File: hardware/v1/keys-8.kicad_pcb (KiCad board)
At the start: 2 copper layers, 13 parts, among them P1 CONN_02X02, P2 CONN_01X03, P3 CONN_01X03, P4 CONN_01X03, SW1 SWITCH_INV, SW2 SWITCH_INV, SW3 SWITCH_INV, SW4 SWITCH_INV, SW5 SWITCH_INV, SW6 SWITCH_INV, SW7 SWITCH_INV, SW8 SWITCH_INV, U1 MCP23017

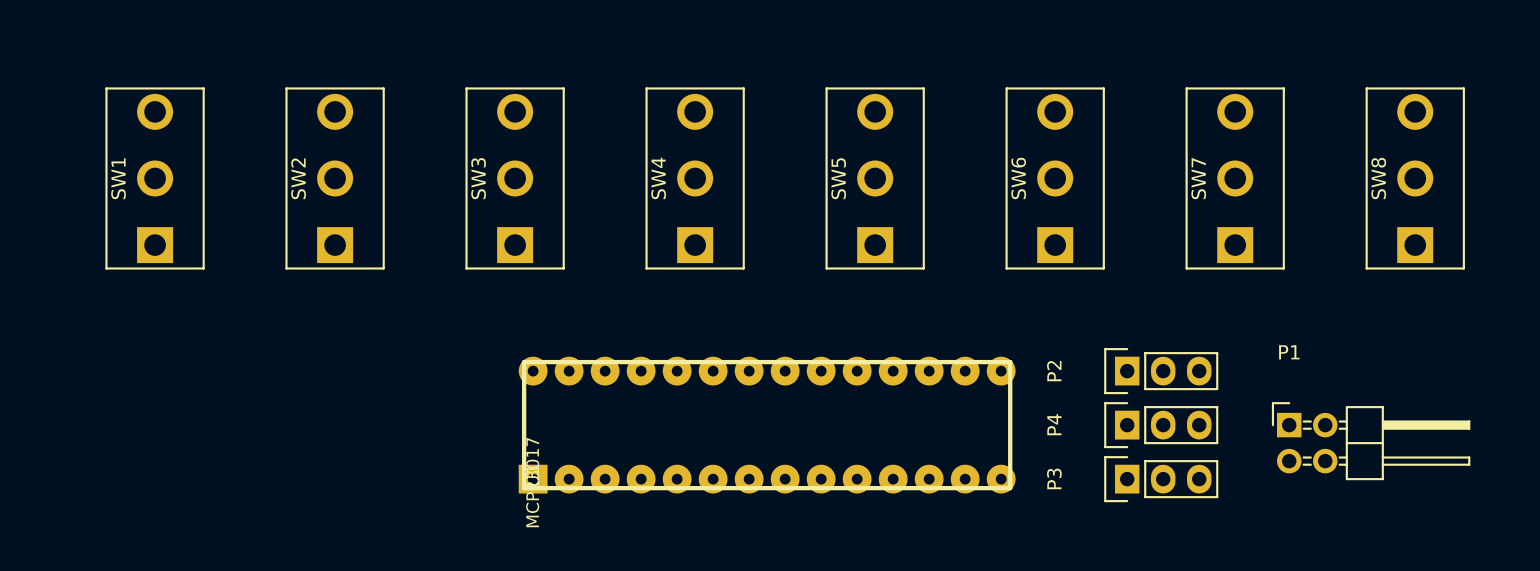
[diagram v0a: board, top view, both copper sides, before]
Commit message: Route keys-8 and generate gerber files.
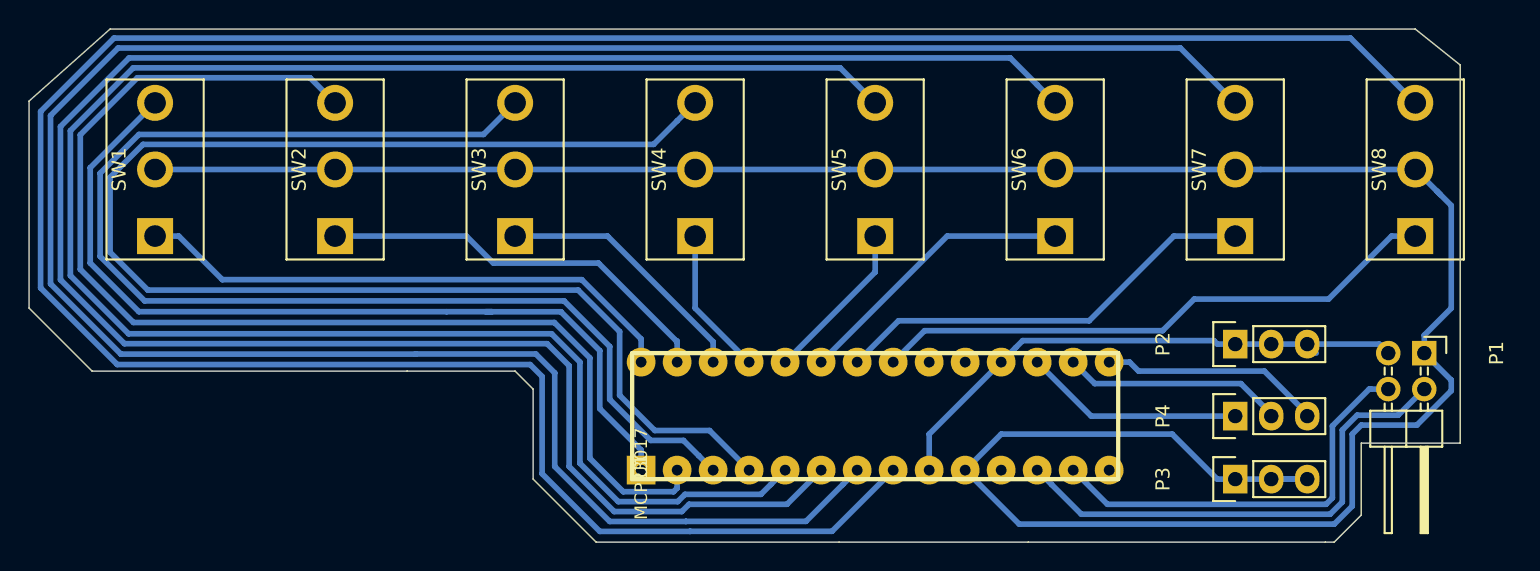
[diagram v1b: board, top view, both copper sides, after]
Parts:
- moved P1 10.8 mm to (229.2, 90.2), turned to 270 degrees
- moved P2 7.85 mm to (215.9, 89.5)
- moved P4 7.65 mm to (215.9, 94.6)
- moved U1 7.65 mm to (174.0, 98.4)
- moved P3 7.62 mm to (215.9, 99.1)
- moved SW1 0.64 mm to (139.7, 77.2)
- moved SW2 0.64 mm to (152.4, 77.2)
- moved SW3 0.64 mm to (165.1, 77.2)
- moved SW4 0.64 mm to (177.8, 77.2)
- moved SW5 0.64 mm to (190.5, 77.2)
- moved SW6 0.64 mm to (203.2, 77.2)
- moved SW7 0.64 mm to (215.9, 77.2)
- moved SW8 0.64 mm to (228.6, 77.2)
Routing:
- net Net-(SW8-Pad3): track 0.00 -> 186.5 mm
- net GND: track 0.00 -> 179.3 mm
- net Net-(SW7-Pad3): track 0.00 -> 168.2 mm
- net Net-(SW6-Pad3): track 0.00 -> 150.1 mm
- net Net-(SW5-Pad3): track 0.00 -> 132.0 mm
- net Net-(SW4-Pad3): track 0.00 -> 102.8 mm
- net Net-(SW3-Pad3): track 0.00 -> 88.9 mm
- net Net-(SW2-Pad3): track 0.00 -> 84.0 mm
- net Net-(SW1-Pad3): track 0.00 -> 61.8 mm
- net Net-(SW8-Pad1): track 0.00 -> 40.5 mm
- net Net-(SW1-Pad1): track 0.00 -> 38.9 mm
- net VDD: track 0.00 -> 38.9 mm
- net /SCK: track 0.00 -> 35.2 mm
- net Net-(SW7-Pad1): track 0.00 -> 30.4 mm
- net /SDA: track 0.00 -> 29.6 mm
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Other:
- board outline added: 101 x 36.2 mm
